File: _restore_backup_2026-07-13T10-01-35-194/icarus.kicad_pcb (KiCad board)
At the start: 4 copper layers, 135.5 x 90 mm, 79 parts, among them CN1 PJ-324, J1 USB_C_Receptacle_USB2.0_16P, J2 SD_Card_Receptacle, J3 LCD ILI9431, J4 JST-PH 2.0mm, Q2 BSS138, Q3 DMG2305UX-7, Q4 2N7002DW_C18208584, SW1 RotaryEncoder_Switch, SW2 SW_Push, SW3 SW_Push, SW4 SS-12D11G5_C49393840, SW5 KH-6X6X9H-ZJ, SW6 KH-6X6X9H-ZJ, SW7 KH-6X6X9H-ZJ, SW8 KH-6X6X9H-ZJ, SW9 KH-6X6X9H-ZJ, U1 ESP32-S3-WROOM-1, U2 AP2112K-3.3, U3 TAD5212IRGER, U4 MCP73831T-2ATI/OT, U7 USBLC6-2SC6

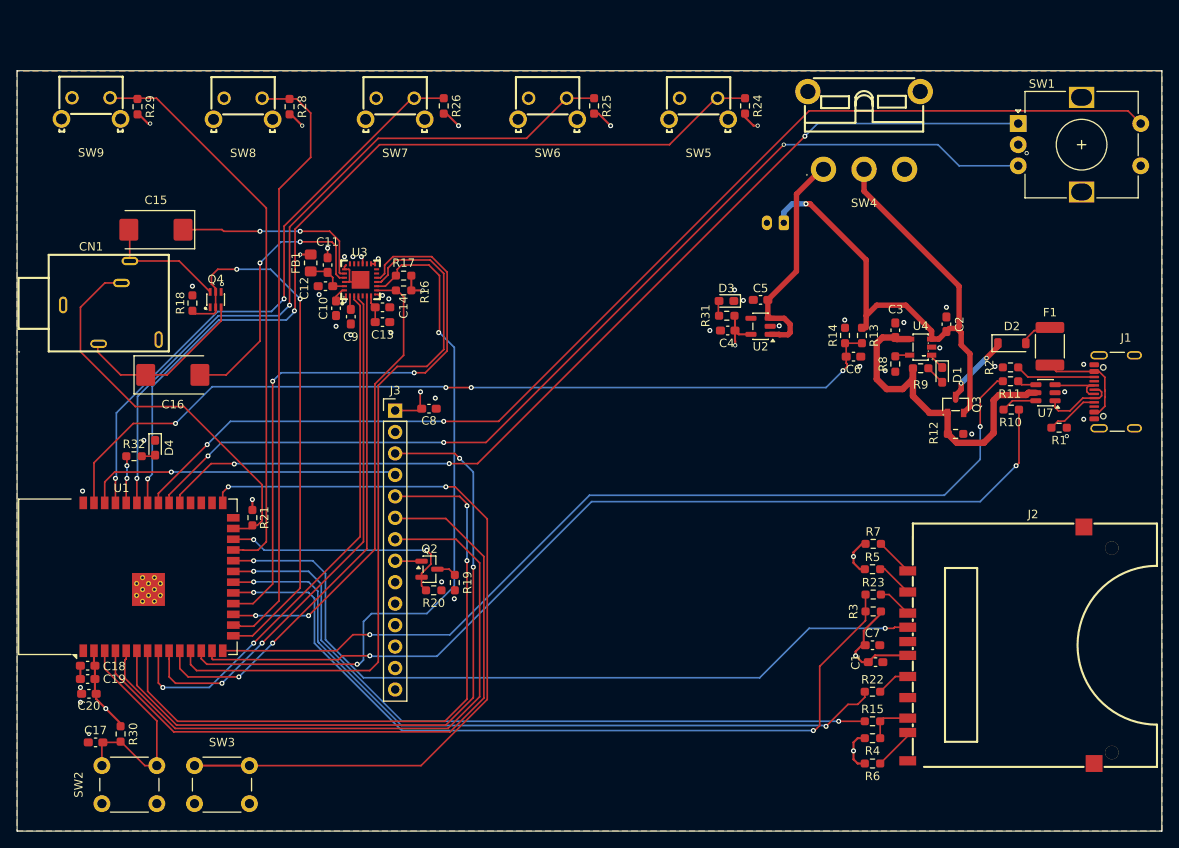
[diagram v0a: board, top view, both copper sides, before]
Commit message: kicad files
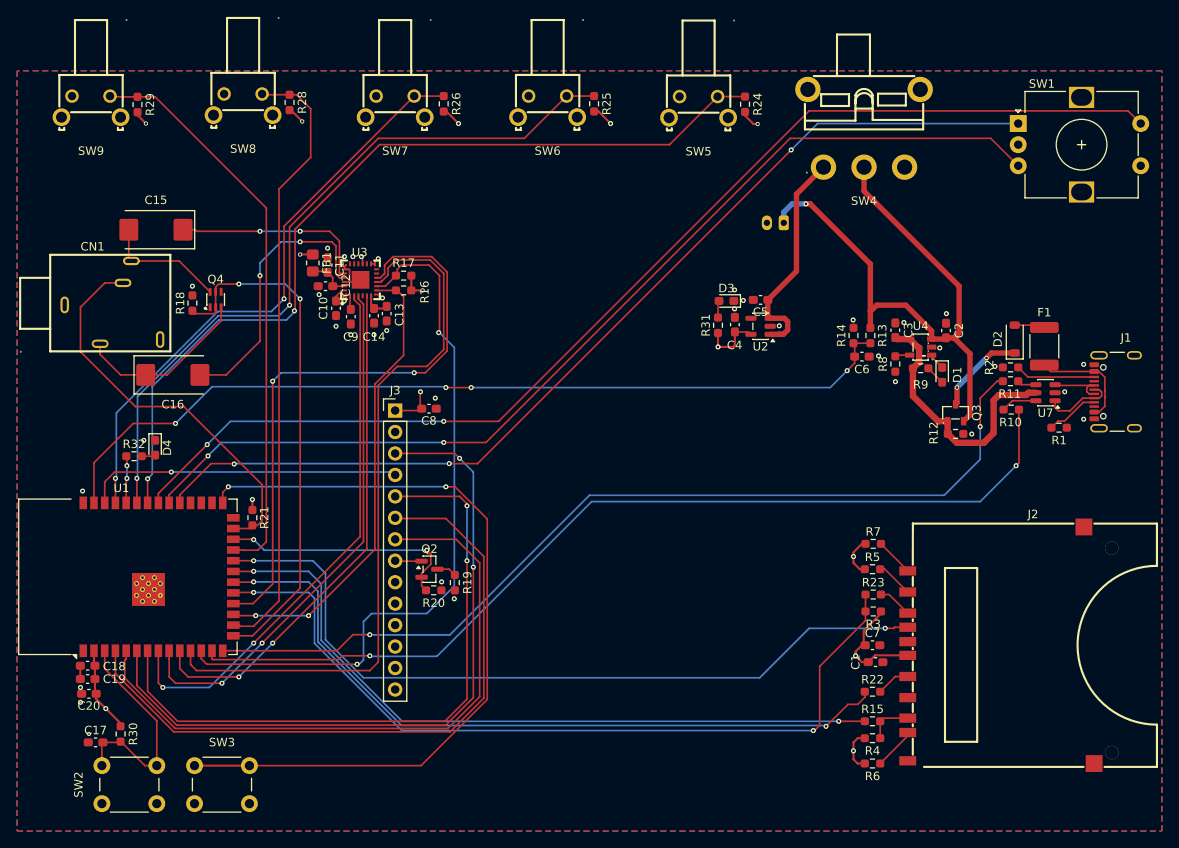
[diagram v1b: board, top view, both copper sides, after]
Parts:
- moved R31 1.53 mm to (188.7, 78.6), turned to 90 degrees
- moved C14 1.41 mm to (148.0, 77.5), turned to -90 degrees
- moved C13 1.12 mm to (149.5, 77.2), turned to 90 degrees
- moved C4 1.10 mm to (190.7, 78.6), turned to 90 degrees
- moved C6 1.00 mm to (205.8, 82.3)
- moved R13 1.00 mm to (206.8, 79.8)
- moved R14 1.00 mm to (204.8, 79.8)
- moved Q3 0.98 mm to (216.8, 89.0)
- moved C2 0.75 mm to (215.7, 79.2)
- moved F1 0.66 mm to (227.3, 81.1)
- moved D2 0.59 mm to (223.8, 80.3), turned to 90 degrees
- moved R28 0.50 mm to (138.0, 52.2)
- moved SW8 0.50 mm to (132.5, 52.5)
- moved R25 0.26 mm to (174.0, 52.4)
- moved SW6 0.26 mm to (168.5, 52.7)
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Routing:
- net VBUS: track 41.4 -> 31.8 mm
- net GPIO3: track 64.3 -> 61.3 mm
- net VSYS: track 8.83 -> 10.6 mm
- net +3.3V: track 61.5 -> 62.9 mm
- net GND: track 11.5 -> 10.5 mm, vias 39 -> 36
- net GPIO39: track 119.7 -> 120.3 mm, vias 3 -> 2
- net GPIO1: track 103.6 -> 104.2 mm
- net VLDOIN: track 26.8 -> 26.3 mm
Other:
- board outline removed
